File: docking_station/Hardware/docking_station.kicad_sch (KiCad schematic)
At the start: 89 parts, among them IC1 VOM1271T, IC2 VOM1271T, IC3 VOM1271T, IC4 VOM1271T, IC5 VOM1271T, J1 WAGO, J2 XT60, J3 Conn_01x05_Pin, J5 SUPPLY+, J6 SUPPLY-, J7 SUPPLY-, K1 RELPOL R40N-3021-85-1024, Q1 SIDR392DP-T1-GE3, Q10 DN2540N8-G, Q11 DN2540N8-G, Q12 2N7002K, Q2 SIDR392DP-T1-GE3, Q3 SIDR392DP-T1-GE3, Q4 SIDR392DP-T1-GE3, Q5 SIDR392DP-T1-GE3, Q6 SIDR392DP-T1-GE3, Q7 SIDR392DP-T1-GE3, Q8 SIDR392DP-T1-GE3, Q9 SIDR392DP-T1-GE3, U1 LTC4357MS8, U2 ACS712xLCTR-20A, U3 L78L05AB, U4 LMV321IYLT, U5 MCP6561T-E/OT, U6 MCP6561T-E/OT

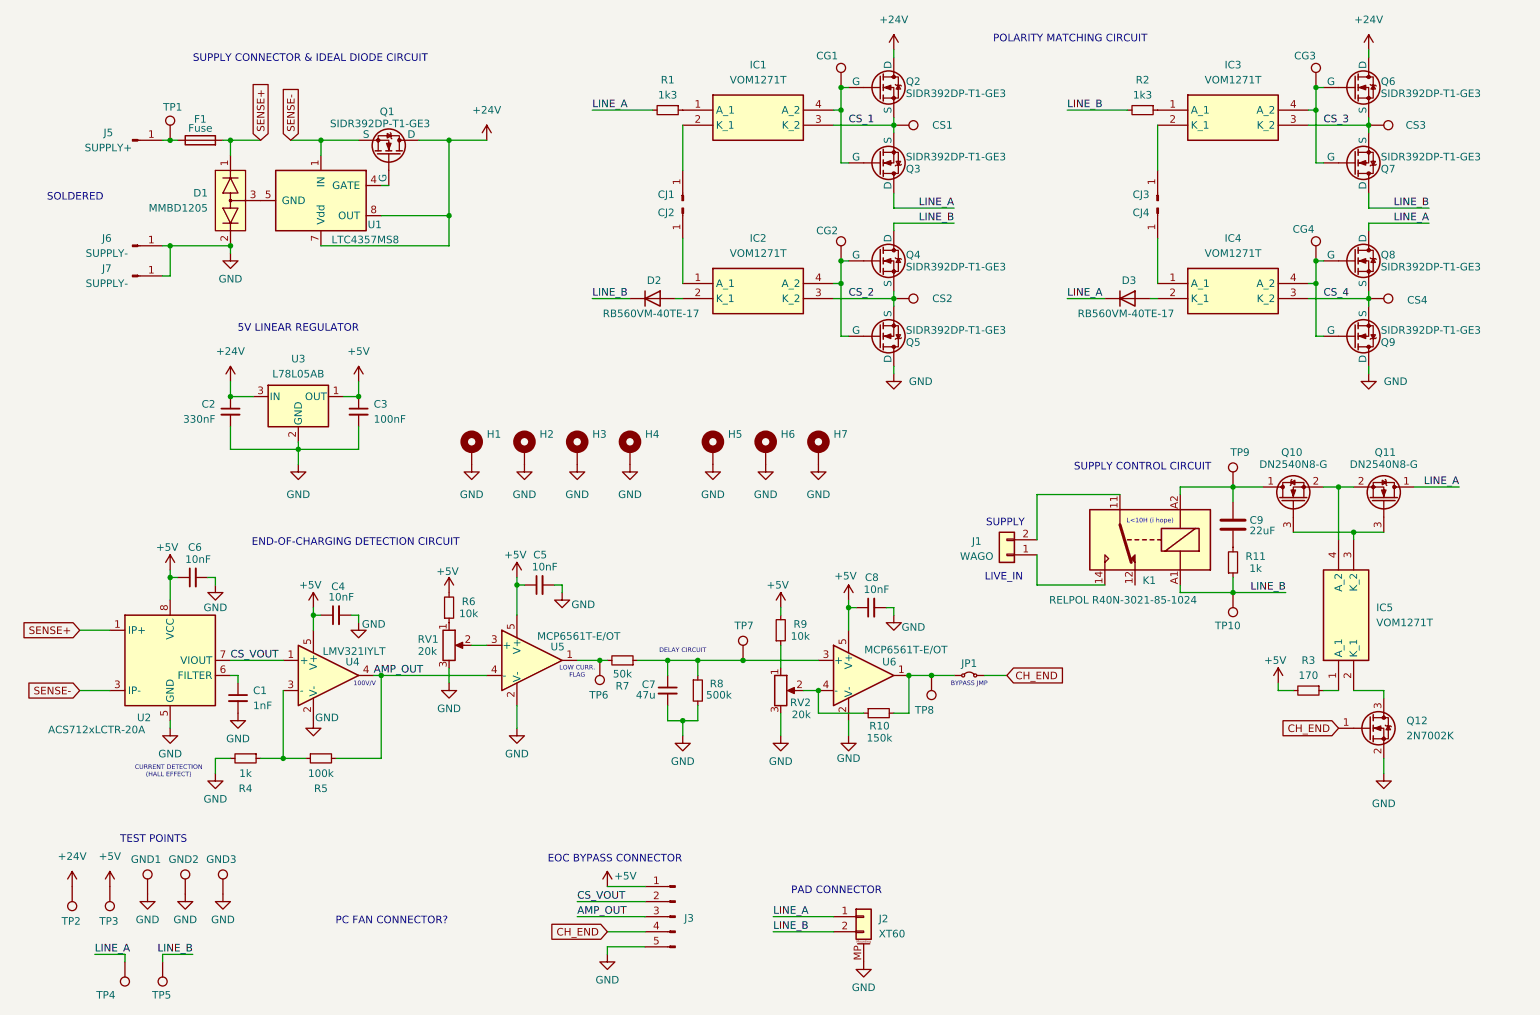
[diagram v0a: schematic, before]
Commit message: big layout updates
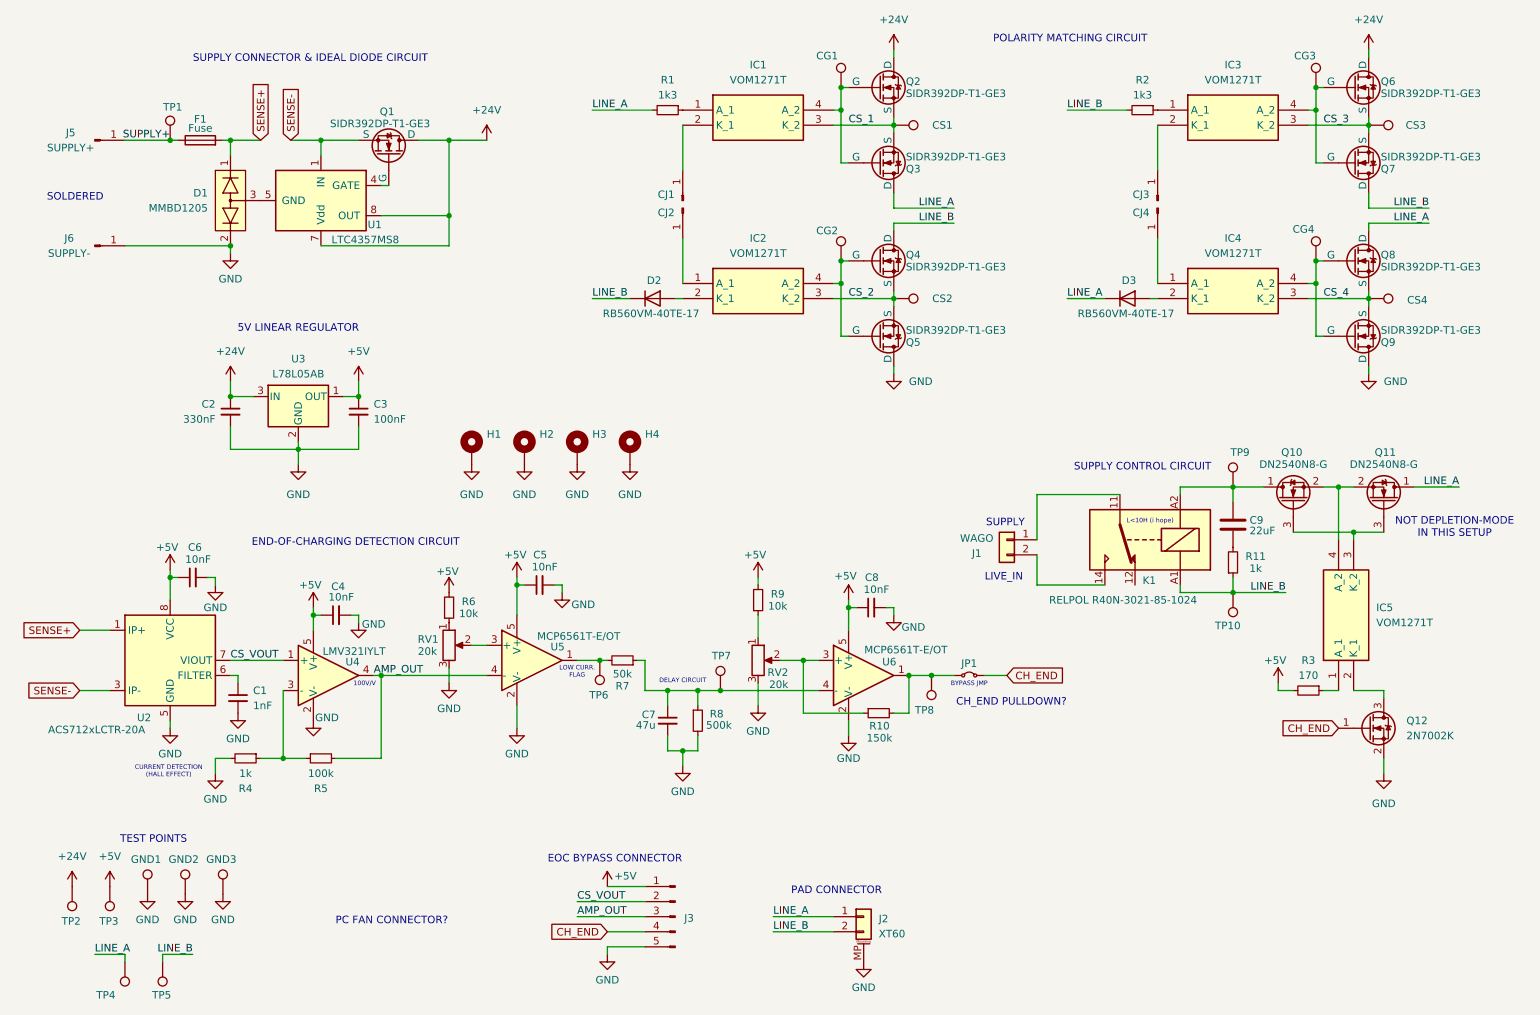
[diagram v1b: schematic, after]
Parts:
- removed H5, H6, H7: MountingHole_Pad, MountingHole:MountingHole_2.2mm_M2_Pad_Via, symbol Mechanical:MountingHole_Pad
- removed J7: SUPPLY-, firo_footprints:14 AWG soldering pad, symbol Connector:Conn_01x01_Pin
- CJ1, CJ2, CJ3, CJ4: footprint Connector_Wire:SolderWire-0.5sqmm_1x01_D0.9mm_OD2.3mm -> firo_footprints:20AWG SMD
- J1: footprint (none) -> firo_footprints:WAGO 2601-3102
- J5, J6: footprint firo_footprints:14 AWG soldering pad -> firo_footprints:14 AWG THT
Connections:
- net at C7.1, R7.1, R8.1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: now also U6.4 (-); no longer U6.3 (+)
- net SUPPLY+: now reaches F1.1, J5.1 (Pin_1), TP1.1
- net at R10.1, RV2.2: now also U6.3 (+); no longer U6.4 (-)
- net at J1.1 (Pin_1): now also K1.11; no longer K1.14
- net at J1.2 (Pin_2): now also K1.14; no longer K1.11
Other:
- note added: "CH_END PULLDOWN?"
- note added: "NOT DEPLETION-MODE IN THIS SETUP"
- moved on the sheet: C7, J1, J5, J6, R8, R9, RV2, TP7
